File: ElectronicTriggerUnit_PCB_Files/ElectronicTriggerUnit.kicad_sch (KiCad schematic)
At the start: 51 parts, among them IC1 MCP1407-E_SN, IC2 ATTINY814-SSF, J2 Conn_01x05, J4 Conn_01x04, M1 Motor_DC, Q1 LC191PTDT, Q2 LKPT30102B-A01, Q3 78-SQRS140ELP, Q4 LC191PTDT, U1 Gnd, U2 12v, U3 GndMotor, U4 Gnd, U5 12v

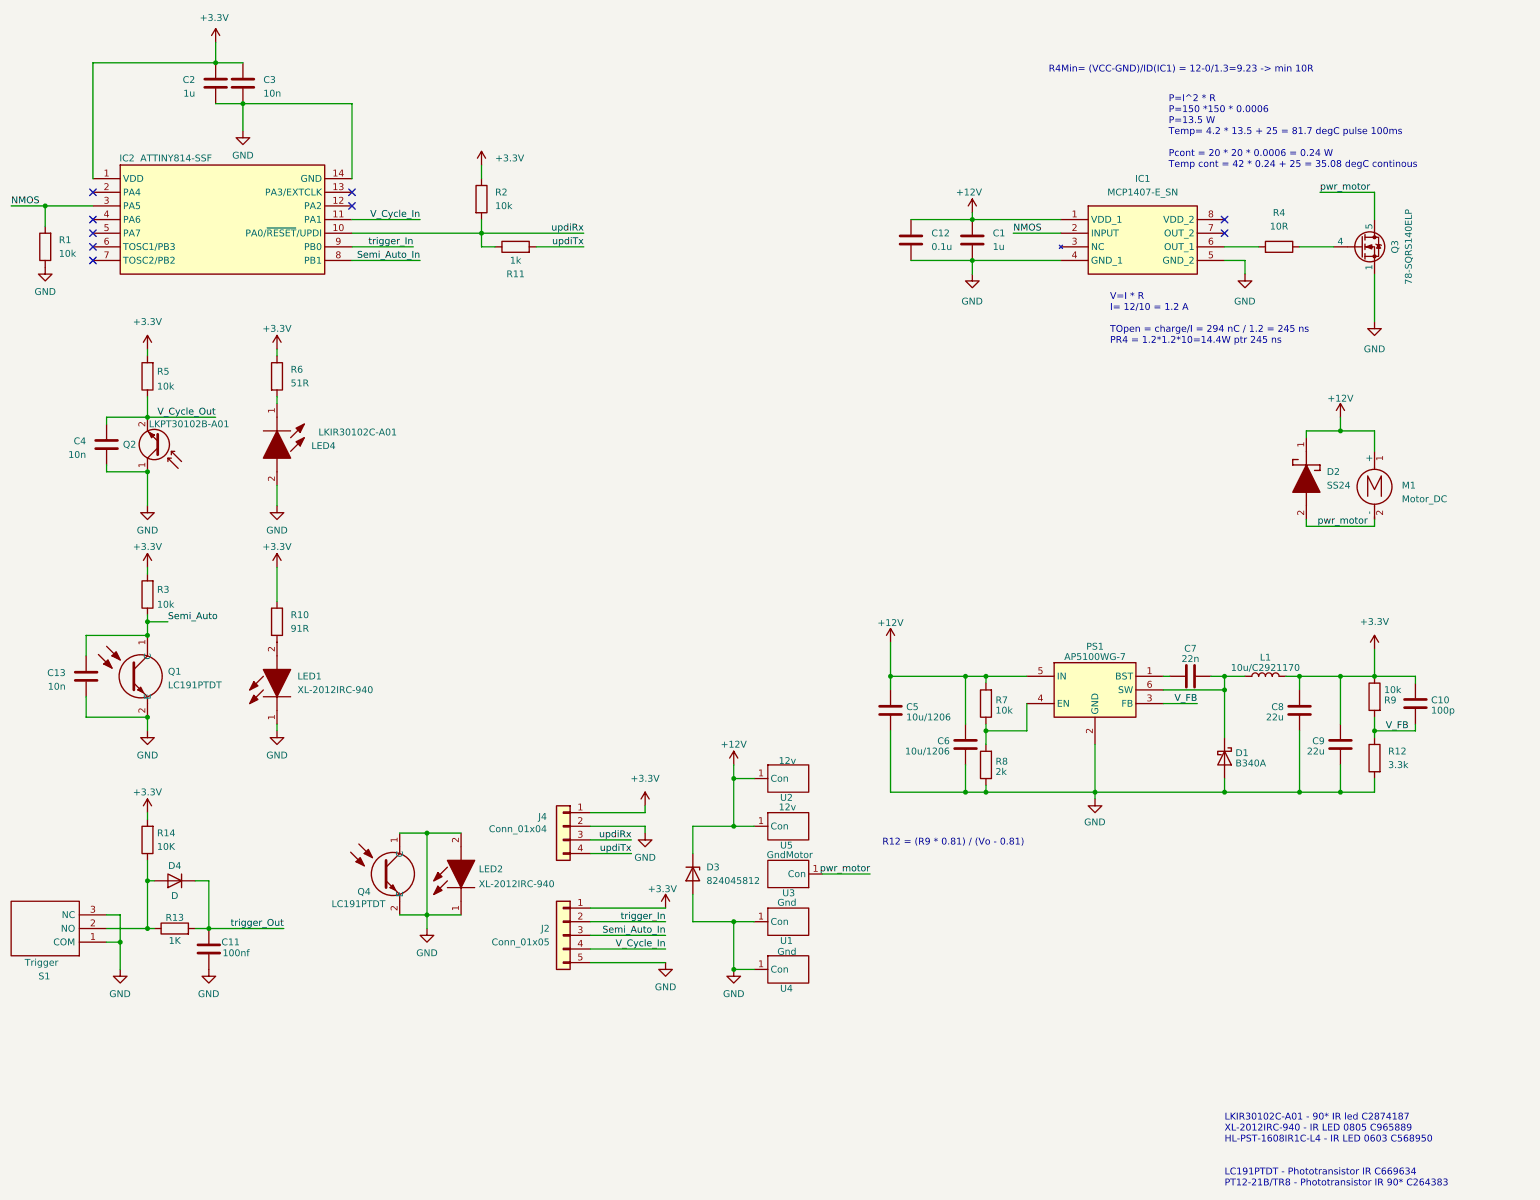
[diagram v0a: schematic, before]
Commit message: changed some parts
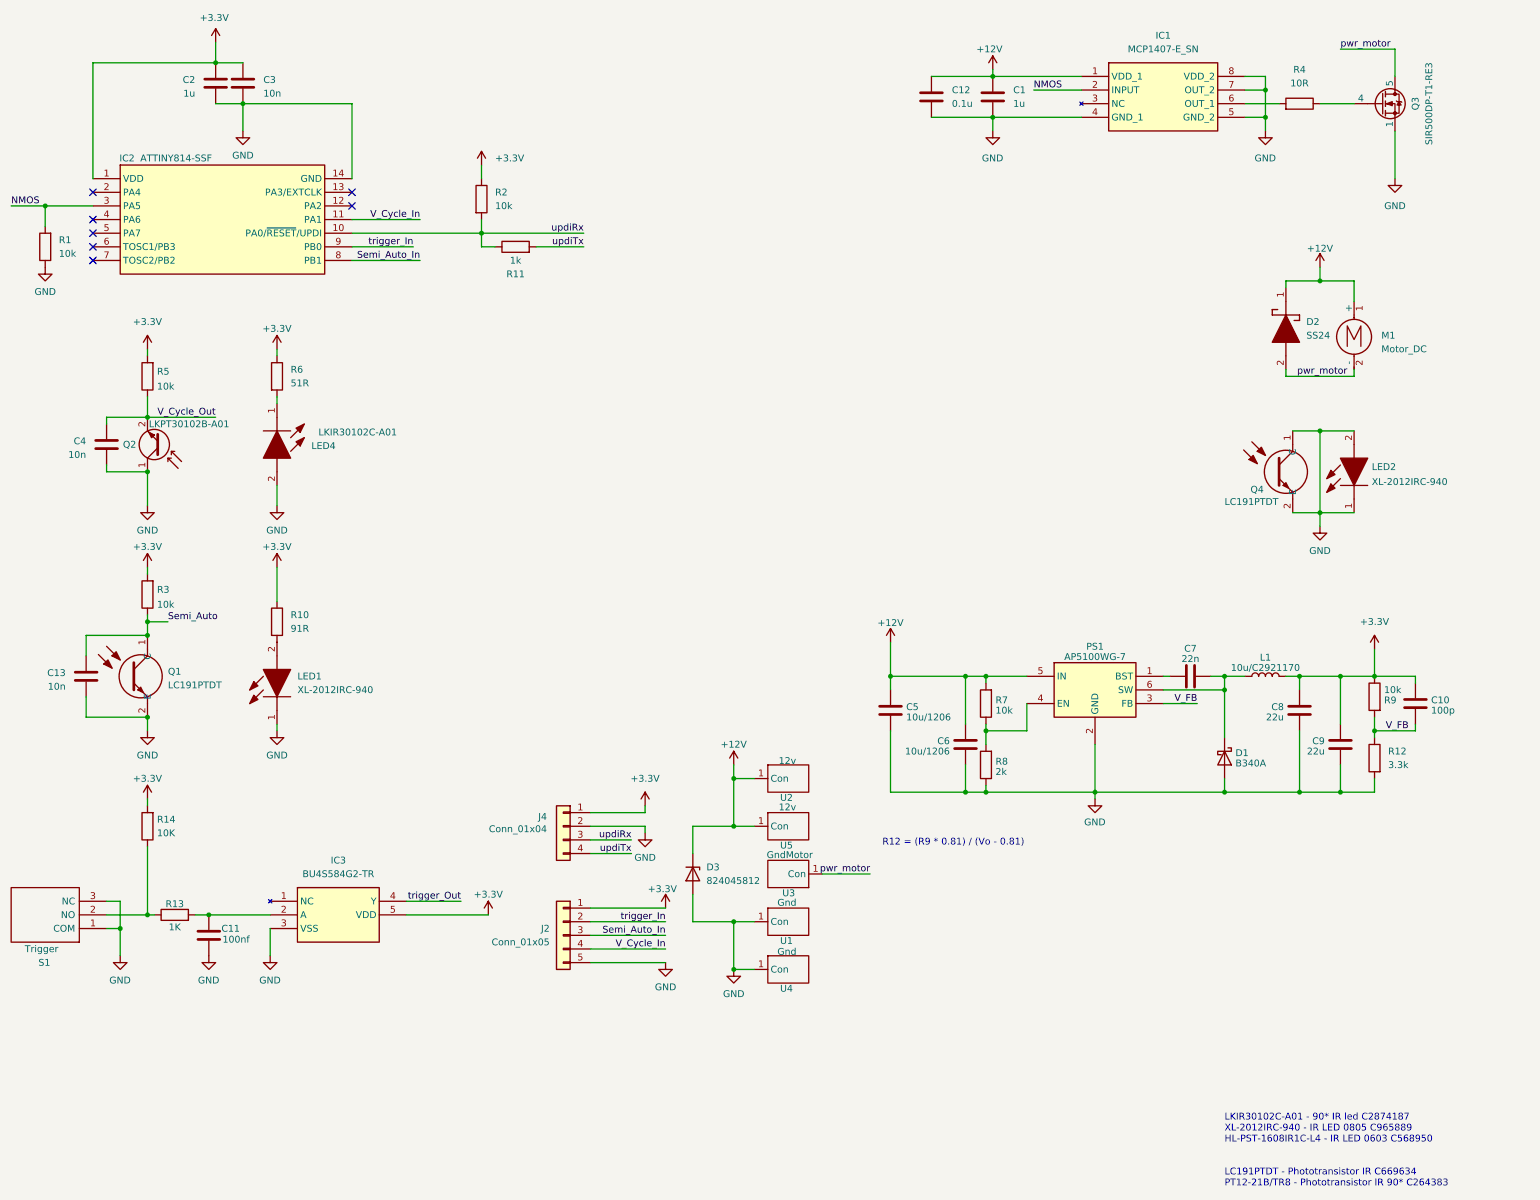
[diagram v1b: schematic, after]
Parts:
- removed D4: D, Diode_SMD:D_0603_1608Metric, symbol Device:D
- added IC3: BU4S584G2-TR, SamacSys:SOT95P280X125-5N, symbol SamacSys:BU4S584G2-TR
- Q3: value 78-SQRS140ELP -> SIR500DP-T1-RE3
- R4: footprint Resistor_SMD:R_0603_1608Metric -> Resistor_SMD:R_1206_3216Metric
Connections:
- net +3.3V: now also IC3.5 (VDD)
- net GND: now also IC1.7 (OUT_2), IC1.8 (VDD_2), IC3.3 (VSS)
- net trigger_Out: now also IC3.4 (Y); no longer C11.2, R13.2
- new net: C11.2, IC3.2 (A), R13.2
- no-connect marks 9 -> 7
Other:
- note removed: "P=I^2 * R P=150 *150 * 0.0006 P=13.5 W Temp= 4.2 * 13.5 + 25 = 81.7 degC pulse 100ms Pcont = 20 * 20 * 0.0006 = 0.24 W Temp cont = 42 * 0.24 + 25 = 35.08 degC continous"
- note removed: "R4Min= (VCC-GND)/ID(IC1) = 12-0/1.3=9.23 -> min 10R"
- note removed: "V=I * R I= 12/10 = 1.2 A TOpen = charge/I = 294 nC / 1.2 = 245 ns PR4 = 1.2*1.2*10=14.4W ptr 245 ns"
- moved on the sheet: C1, C11, C12, D2, IC1, LED2, M1, Q3, Q4, R13, R14, R4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
